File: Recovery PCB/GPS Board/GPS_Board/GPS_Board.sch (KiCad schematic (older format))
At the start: 11 parts, among them J1 XT30-M, J2 XT30-M, U1 Teensy4.1

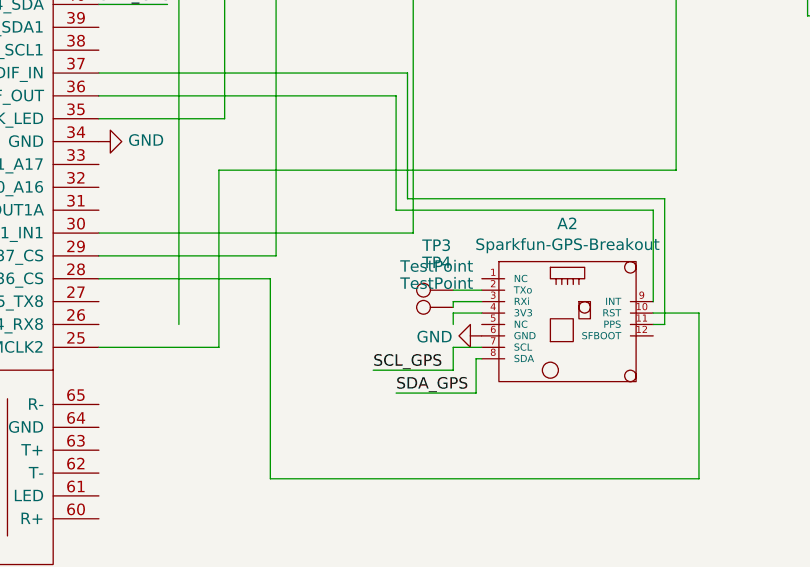
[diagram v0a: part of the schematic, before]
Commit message: GPS
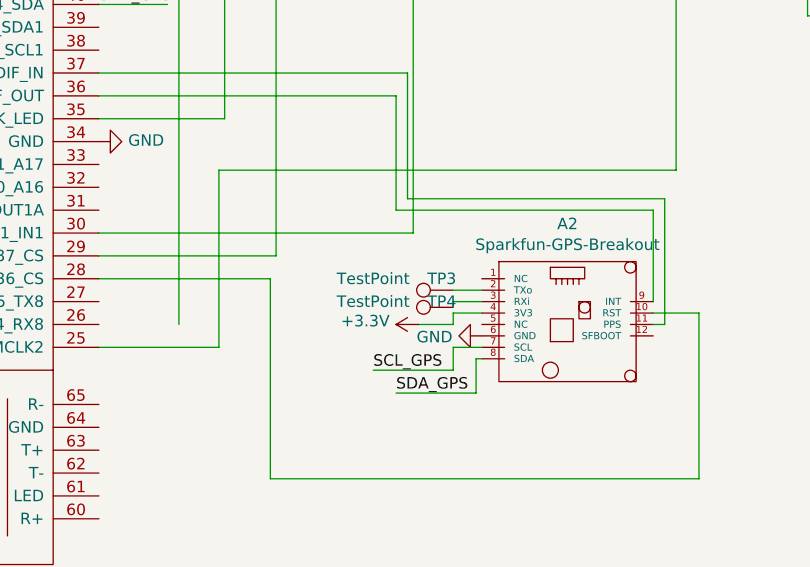
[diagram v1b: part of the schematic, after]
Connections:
- net labels added: +3.3V
- wire segments 74 -> 75
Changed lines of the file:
@@
 U 1 1 61AB8223
 P 5550 3450
-F 0 "TP3" V 5745 3522 50  0000 C CNN
-F 1 "TestPoint" V 5654 3522 50  0000 C CNN
+F 0 "TP3" V 5600 3500 50  0000 C CNN
+F 1 "TestPoint" V 5600 3800 50  0000 C CNN
 F 2 "TestPoint:TestPoint_Pad_D1.5mm" H 5750 3450 50  0001 C CNN
 F 3 "~" H 5750 3450 50  0001 C CNN
@@
 U 1 1 61AB9396
 P 5550 3525
-F 0 "TP4" V 5745 3597 50  0000 C CNN
-F 1 "TestPoint" V 5654 3597 50  0000 C CNN
+F 0 "TP4" V 5575 3575 50  0000 C CNN
+F 1 "TestPoint" V 5575 3875 50  0000 C CNN
 F 2 "TestPoint:TestPoint_Pad_D1.5mm" H 5750 3525 50  0001 C CNN
 F 3 "~" H 5750 3525 50  0001 C CNN
@@
 	0    1    1    0
 $EndComp
-Wire Wire Line
-	5675 3550 5550 3550
-Wire Wire Line
-	5550 3550 5550 3600
 Wire Wire Line
 	4350 3600 4350 1600
@@
 $EndComp
 Wire Wire Line
-	6425 3500 6425 3100
-Wire Wire Line
-	6425 3100 5300 3100
-Wire Wire Line
 	5300 3100 5300 2600
 Wire Wire Line
@@
 Wire Wire Line
 	4000 2100 4300 2100
+Wire Wire Line
+	5550 3550 5675 3550
+Wire Wire Line
+	5550 3550 5550 3600
+Wire Wire Line
+	5550 3600 5400 3600
+$Comp
+L power:+3.3V #PWR?
+U 1 1 625F178F
+P 5400 3600
+F 0 "#PWR?" H 5400 3450 50  0001 C CNN
+F 1 "+3.3V" V 5415 3728 50  0000 L CNN
+F 2 "" H 5400 3600 50  0001 C CNN
+F 3 "" H 5400 3600 50  0001 C CNN
+	1    5400 3600
+	0    -1   -1   0
+$EndComp
+Wire Wire Line
+	6425 3500 6425 3100
+Wire Wire Line
+	6425 3100 5300 3100
 $EndSCHEMATC
